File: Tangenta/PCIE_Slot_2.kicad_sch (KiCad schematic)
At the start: 5 parts, among them J10 1-2199230-5

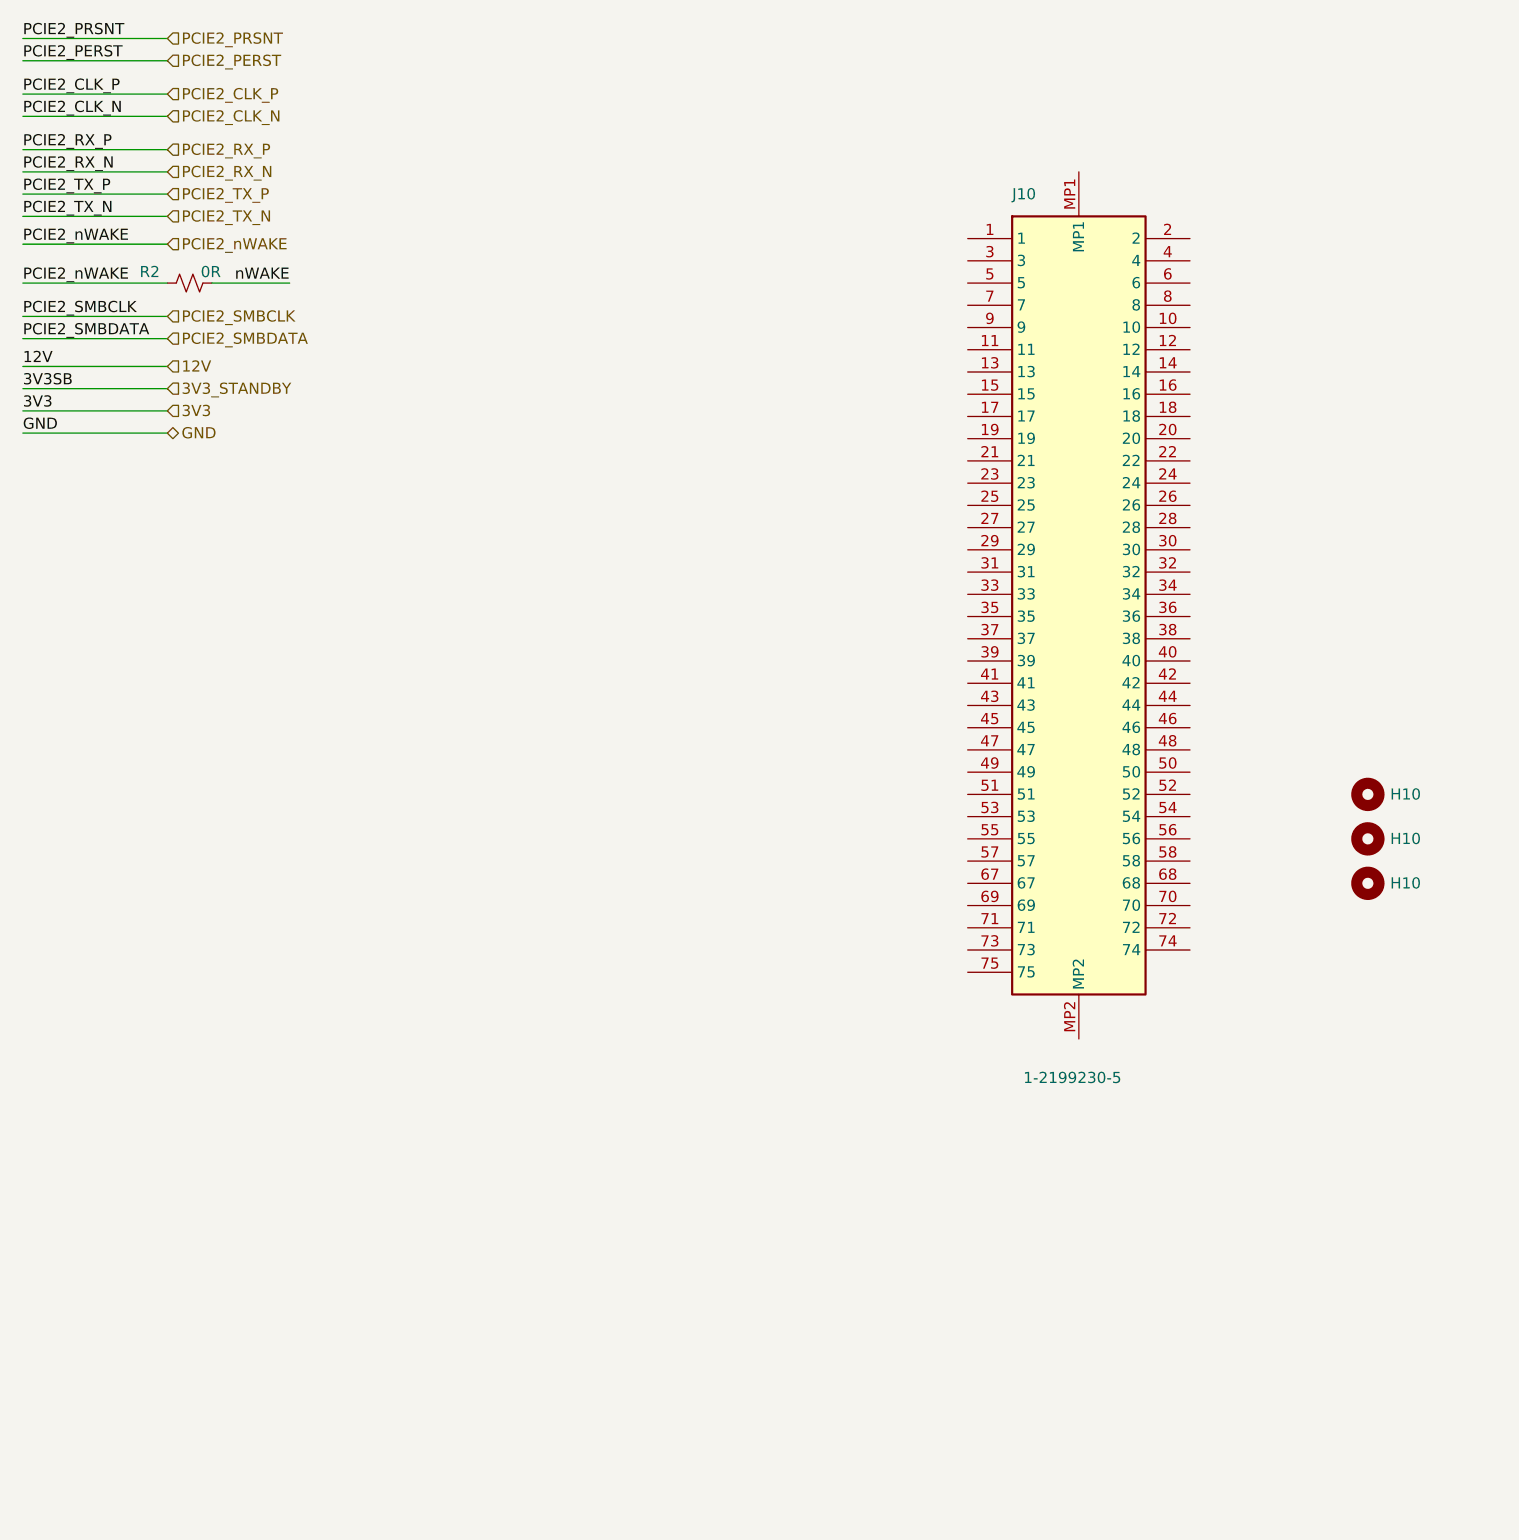
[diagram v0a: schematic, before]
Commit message: ...
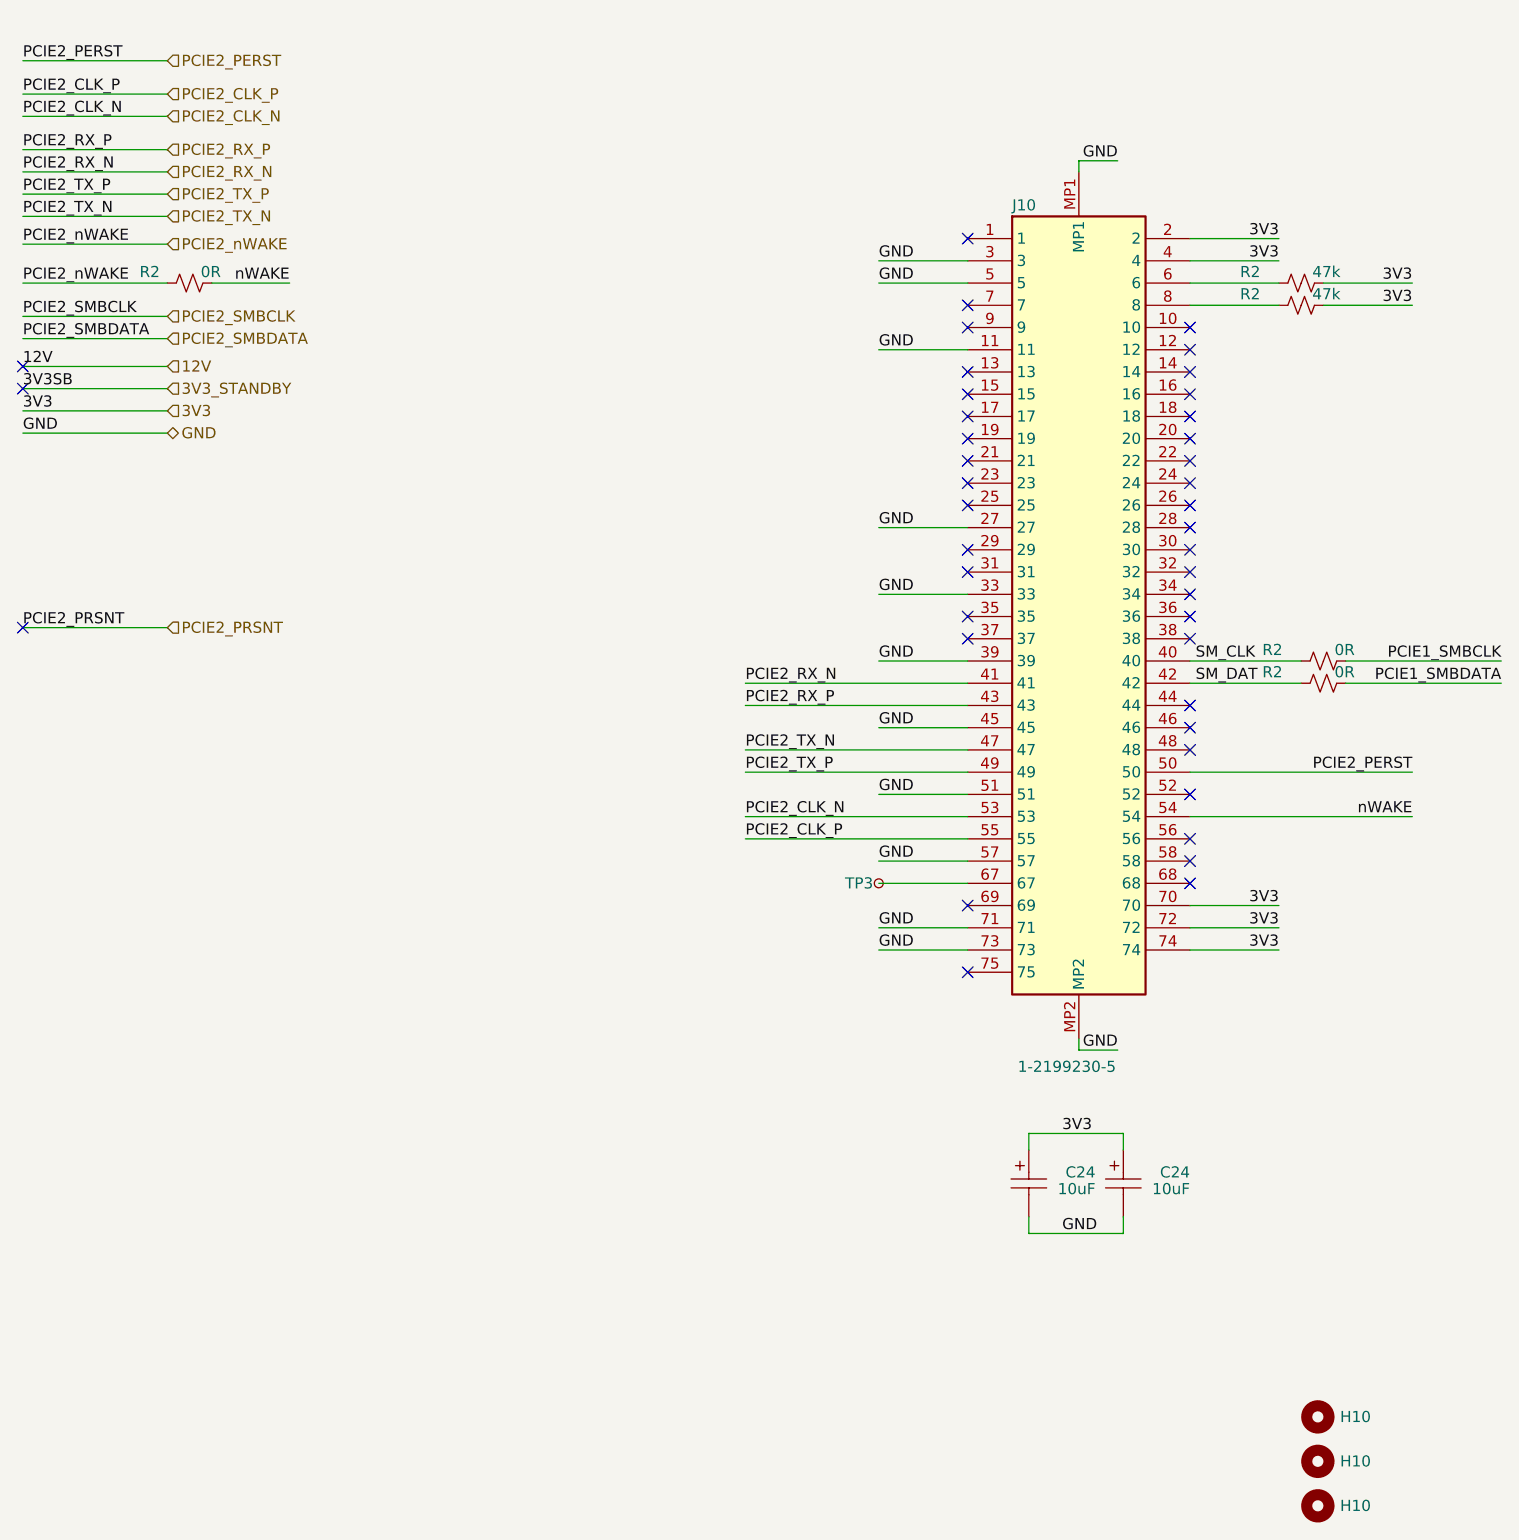
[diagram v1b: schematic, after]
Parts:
- added C24 (x2): 10uF, CAP_TANTAL_A:CAP_TANTAL_A, symbol CAP_TANTAL_A:CA45-A-6_3V-47UF-K
- added R2 (x2): 47k, Resistor_SMD:R_0402_1005Metric, symbol Device:R_Small_US
- added R2 (x2): 0R, Resistor_SMD:R_0402_1005Metric, symbol Device:R_Small_US
- added TP3: TestPoint_Small, TestPoint:TestPoint_Pad_1.0x1.0mm, symbol Connector:TestPoint_Small
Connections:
- net 3V3: now also J10.2, J10.4, J10.70, J10.72, J10.74, C24.1, C24.1, R2.1, R2.1
- net GND: now also J10.11, J10.27, J10.3, J10.33, J10.39, J10.45, J10.5, J10.51, J10.57, J10.71, J10.73, J10.MP1, J10.MP2, C24.2, C24.2
- net PCIE2_CLK_N: now also J10.53
- net PCIE2_CLK_P: now also J10.55
- net PCIE2_PERST: now also J10.50
- net PCIE2_RX_N: now also J10.41
- net PCIE2_RX_P: now also J10.43
- net PCIE2_TX_N: now also J10.47
- net PCIE2_TX_P: now also J10.49
- net nWAKE: now also J10.54
- net SM_CLK: now reaches J10.40
- net SM_CLK: now also R2.2
- net SM_DAT: now reaches J10.42
- net SM_DAT: now also R2.2
- net at J10.6: now also R2.2
- net at J10.67: now also TP3.1
- net at J10.8: now also R2.2
- new net PCIE1_SMBCLK: R2.1
- new net PCIE1_SMBDATA: R2.1
- no-connect marks 0 -> 41
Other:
- moved on the sheet: H10
